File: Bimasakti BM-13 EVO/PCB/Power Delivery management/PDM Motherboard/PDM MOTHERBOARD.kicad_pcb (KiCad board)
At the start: 2 copper layers, 86.5 x 81.4 mm, 45 parts

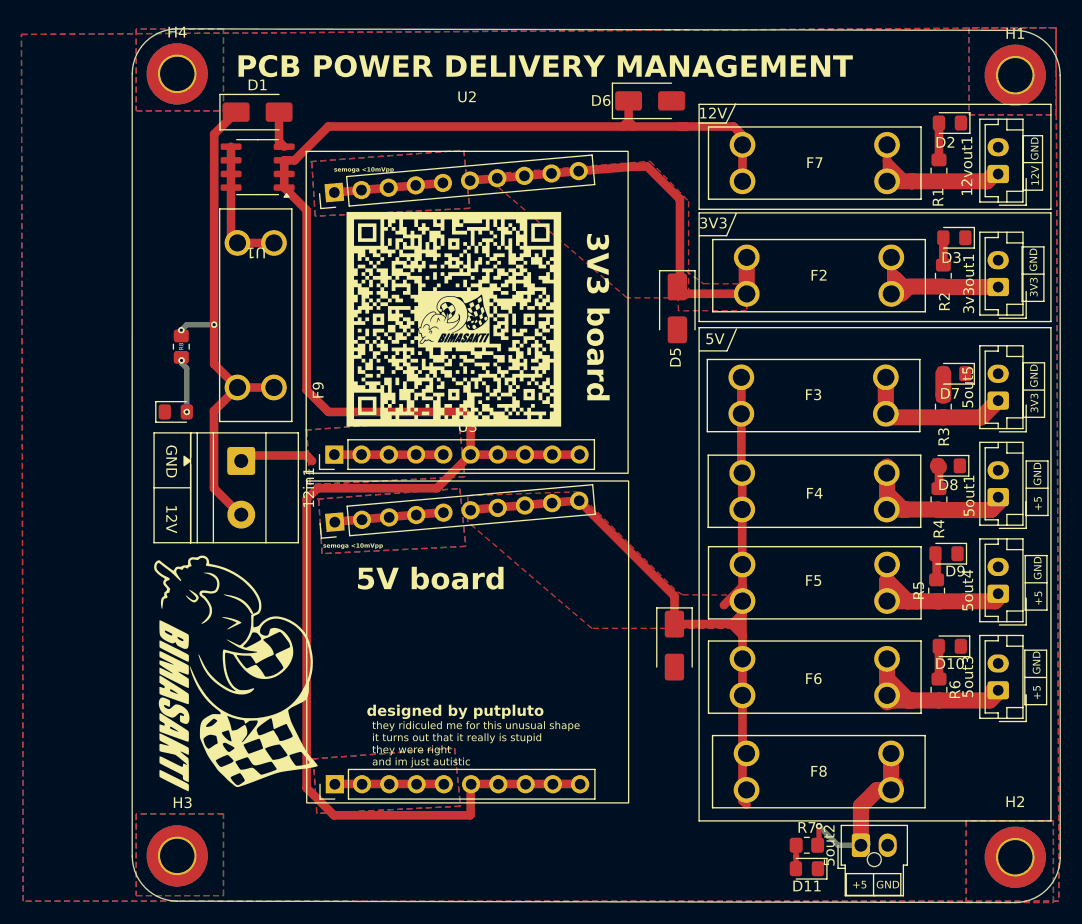
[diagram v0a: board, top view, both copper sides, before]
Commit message: tv dengan pdm kecil
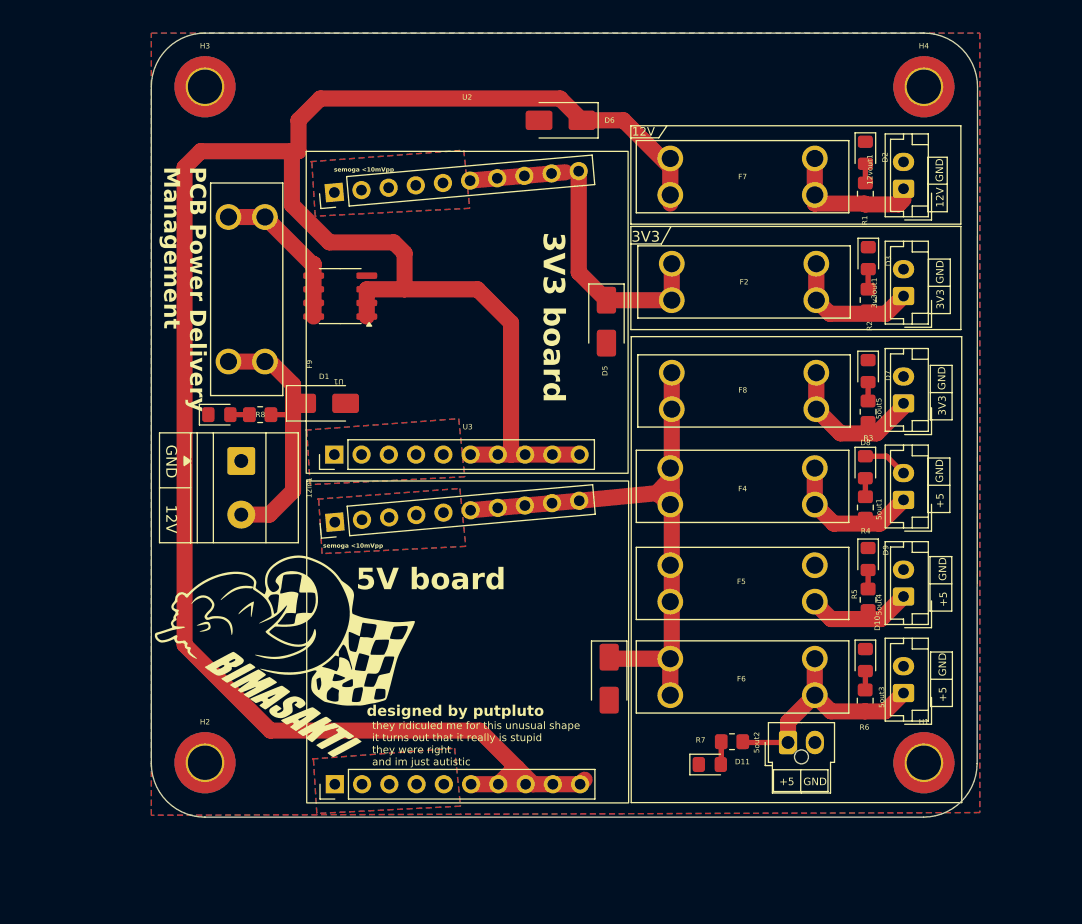
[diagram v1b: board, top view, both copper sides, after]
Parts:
- removed F3: 3557-2, 0_FUSE:0_FUSE_3557-2
- removed the G*** at (101.1, 42.2)
- moved H2 76.0 mm to (77.9, 83.5)
- moved H3 71.7 mm to (77.9, 20.5)
- moved H4 69.6 mm to (144.9, 20.5)
- moved H1 64.6 mm to (144.9, 83.5)
- moved F8 36.2 mm to (128.1, 48.8)
- moved D1 27.8 mm to (89.0, 50.0)
- moved U1 14.3 mm to (90.4, 47.5)
- moved D11 13.3 mm to (124.9, 83.7), turned to 0 degrees
- moved R7 11.9 mm to (127.0, 81.5)
- moved 5out2 11.7 mm to (132.2, 81.6)
- moved R8 9.70 mm to (83.0, 51.1), turned to 180 degrees
- moved 12vout1 8.93 mm to (143.0, 30.0)
- moved 3v3out1 8.86 mm to (143.0, 40.0)
- moved 5out1 8.83 mm to (143.0, 59.0)
- moved 5out3 8.83 mm to (143.0, 77.0)
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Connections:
- 5out2 pad 1: Net-(5out2-Pin_1) -> /5v_f3
- 5out3 pad 1: Net-(5out3-Pin_1) -> /5v_f3
- F6 pad 2_1: Net-(5out3-Pin_1) -> /5v_f3
- F6 pad 2_2: Net-(5out3-Pin_1) -> /5v_f3
- F8 pad 2_1: Net-(5out2-Pin_1) -> Net-(5out5-Pin_1)
- F8 pad 2_2: Net-(5out2-Pin_1) -> Net-(5out5-Pin_1)
- H3 pad 1: GND -> (no net)
- H4 pad 1: GND -> (no net)
- R6 pad 1: Net-(5out3-Pin_1) -> /5v_f3
- R7 pad 1: Net-(5out2-Pin_1) -> /5v_f3
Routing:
- net GND: track 49.9 -> 4.21 mm
- net 12tobuck: track 178.4 -> 211.6 mm
- net Net-(12in1-Pin_2): track 48.4 -> 24.7 mm, vias 2 -> 0
- net /5v_f3: track 0.00 -> 22.7 mm
- net Net-(5out2-Pin_1): track 19.7 -> 0.00 mm, vias 1 -> 0
- net Net-(5out3-Pin_1): track 18.6 -> 0.00 mm
- net 5Vin: track 74.9 -> 58.2 mm
- net Net-(5out4-Pin_1): track 18.1 -> 9.77 mm
- net 3Vin: track 38.5 -> 31.5 mm
- net Net-(3v3out1-Pin_1): track 19.7 -> 12.7 mm
- net Net-(12vout1-Pin_1): track 16.9 -> 11.9 mm
- net Net-(5out1-Pin_1): track 16.8 -> 13.3 mm
- net Net-(D12-A): track 4.99 -> 1.78 mm, vias 2 -> 0
- net Net-(U1-D): track 12.6 -> 14.6 mm
- net Net-(D2-A): track 3.43 -> 1.79 mm
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- removed copper zone on F.Cu, net 3Vin
- removed copper zone on F.Cu, net 5Vin
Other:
- board size 86.5 x 81.4 mm -> 77 x 73.1 mm
- board text added: "PCB Power Delivery Management"
- board text removed: "5V"
- board text removed: "PCB POWER DELIVERY MANAGEMENT"
